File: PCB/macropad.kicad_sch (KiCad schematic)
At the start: 11 parts, among them SW10 SW_Push, SW11 SW_Push, SW12 SW_Push, SW2 RotaryEncoder_Switch, SW3 SW_Push, SW4 SW_Push, SW5 SW_Push, SW6 SW_Push, SW7 SW_Push, SW8 SW_Push, U1 XIAO-RP2040-DIP

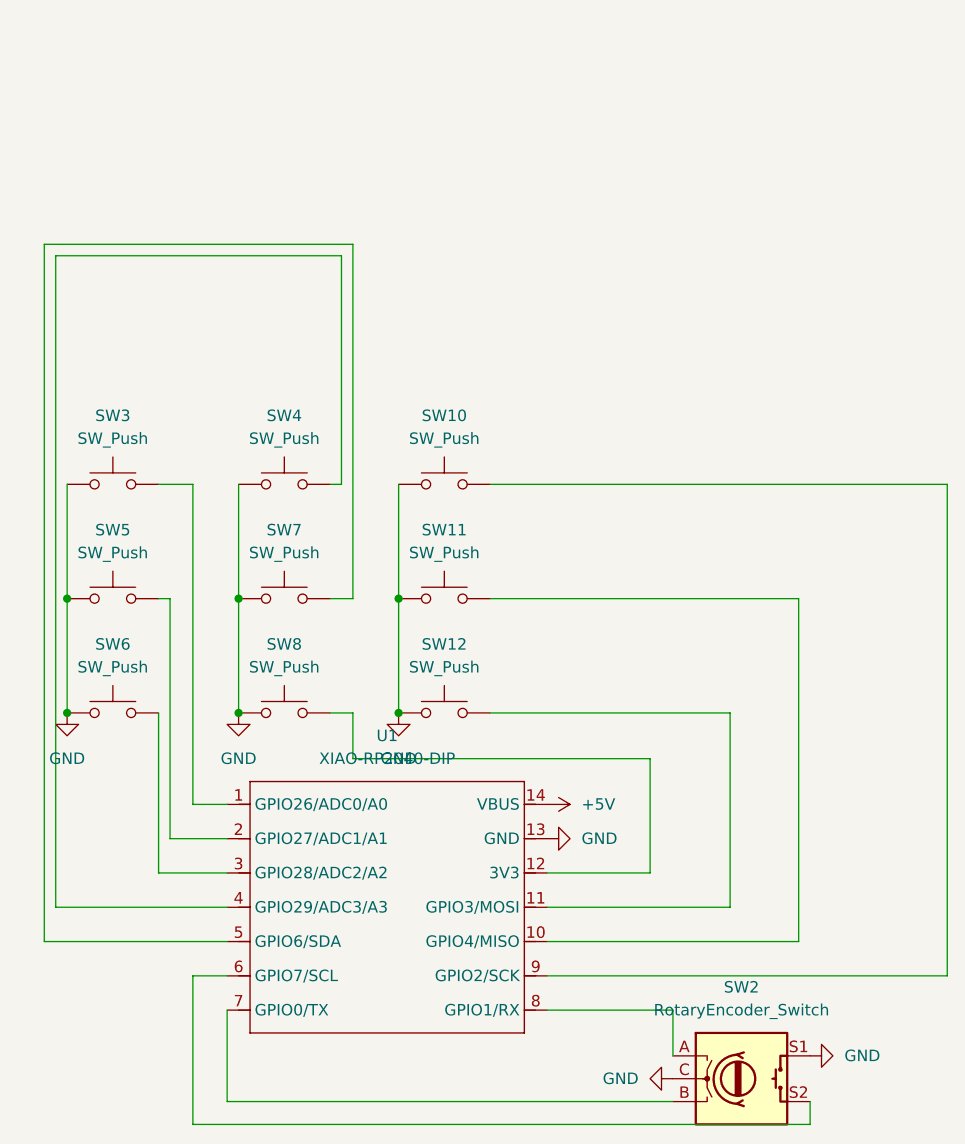
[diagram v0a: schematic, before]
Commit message: Redesign
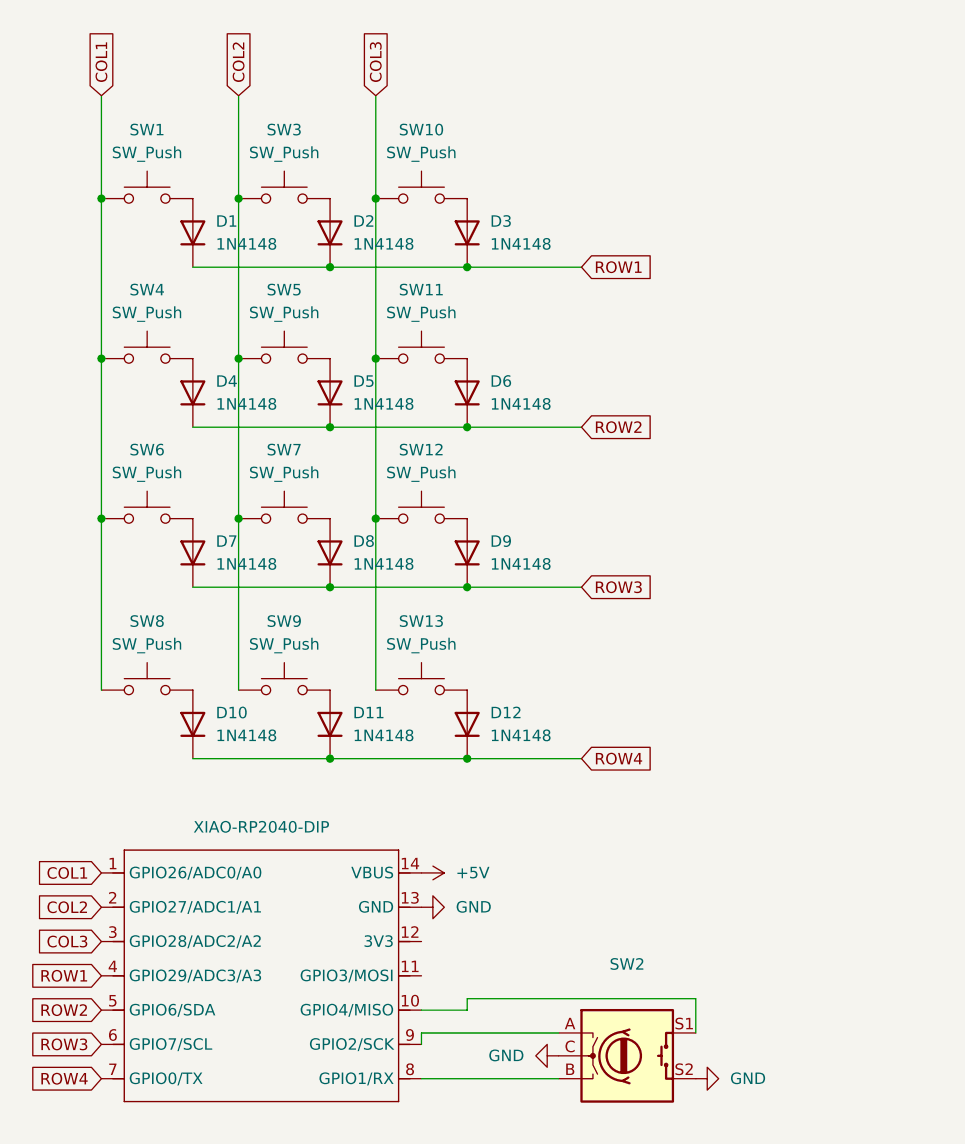
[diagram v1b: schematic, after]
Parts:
- added D1, D10, D11, D12, D2, D3, D4, D5, D6, D7, D8, D9: 1N4148, Diode_THT:D_DO-35_SOD27_P7.62mm_Horizontal, symbol Diode:1N4148
- added SW1, SW13, SW9: SW_Push, Button_Switch_Keyboard:SW_Cherry_MX_1.00u_PCB, symbol Switch:SW_Push
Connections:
- net GND: now also SW2.S2; no longer SW10.1, SW11.1, SW12.1, SW2.S1, SW3.1, SW4.1, SW5.1, SW6.1, SW7.1, SW8.1
- net at SW6.2: now also D7.2 (A); no longer U1.3 (GPIO28/ADC2/A2)
- net at U1.11 (GPIO3/MOSI): no longer SW12.2
- net at SW2.A: now also U1.9 (GPIO2/SCK); no longer U1.8 (GPIO1/RX)
- net at SW2.B: now also U1.8 (GPIO1/RX); no longer U1.7 (GPIO0/TX)
- net ROW3: now reaches U1.6 (GPIO7/SCL)
- net ROW3: now also D7.1 (K), D8.1 (K), D9.1 (K); no longer SW2.S2
- net at SW3.2: now also D2.2 (A); no longer U1.1 (GPIO26/ADC0/A0)
- net at U1.10 (GPIO4/MISO): now also SW2.S1; no longer SW11.2
- net at U1.12 (3V3): no longer SW8.2
- net at SW5.2: now also D5.2 (A); no longer U1.2 (GPIO27/ADC1/A1)
- net at SW4.2: now also D4.2 (A); no longer U1.4 (GPIO29/ADC3/A3)
- net at SW7.2: now also D8.2 (A); no longer U1.5 (GPIO6/SDA)
- net at SW10.2: now also D3.2 (A); no longer U1.9 (GPIO2/SCK)
- new net: D11.2 (A), SW9.2
- new net: D1.2 (A), SW1.2
- new net: D6.2 (A), SW11.2
- new net: D9.2 (A), SW12.2
- new net: D10.2 (A), SW8.2
- new net: D12.2 (A), SW13.2
- new net COL1: SW1.1, SW4.1, SW6.1, SW8.1, U1.1 (GPIO26/ADC0/A0)
- new net COL2: SW3.1, SW5.1, SW7.1, SW9.1, U1.2 (GPIO27/ADC1/A1)
- new net COL3: SW10.1, SW11.1, SW12.1, SW13.1, U1.3 (GPIO28/ADC2/A2)
- new net ROW1: D1.1 (K), D2.1 (K), D3.1 (K), U1.4 (GPIO29/ADC3/A3)
- new net ROW2: D4.1 (K), D5.1 (K), D6.1 (K), U1.5 (GPIO6/SDA)
- new net ROW4: D10.1 (K), D11.1 (K), D12.1 (K), U1.7 (GPIO0/TX)
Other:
- moved on the sheet: SW2
